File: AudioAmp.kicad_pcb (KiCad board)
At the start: 2 copper layers, 60.1 x 56.5 mm, 10 parts, among them J1 Conn_01x02, J2 Conn_01x02, J3 Conn_01x02, U1 LM386

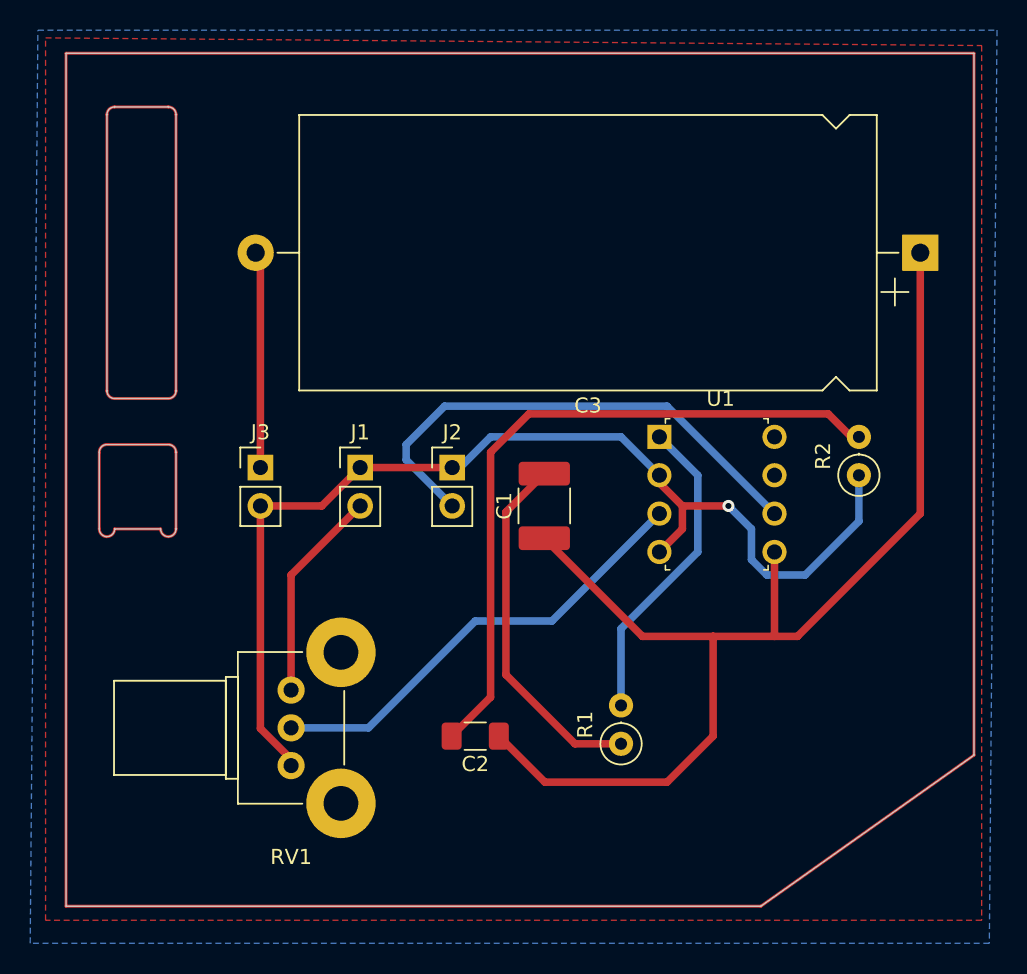
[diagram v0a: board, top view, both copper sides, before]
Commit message: Edits based on what I see
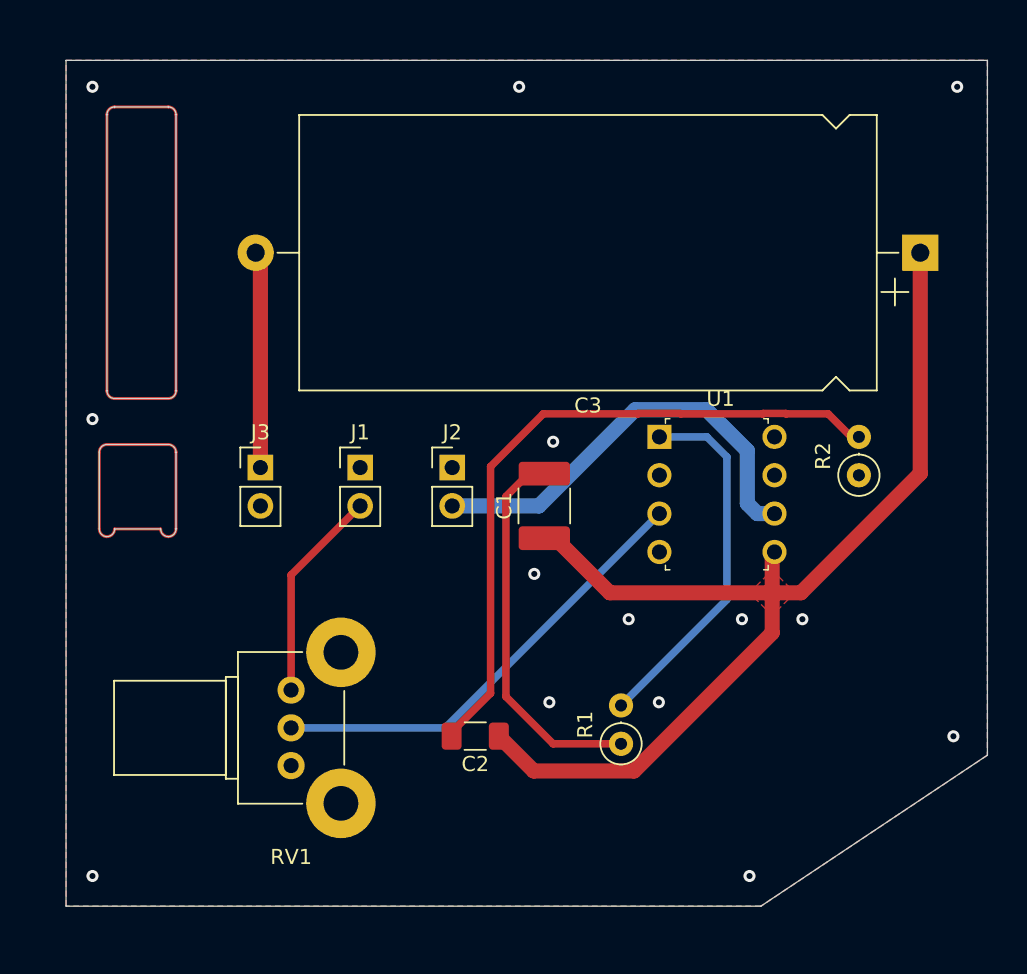
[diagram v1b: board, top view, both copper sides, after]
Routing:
- net GND: track 73.0 -> 0.94 mm, vias 1 -> 14
- net Net-(J2-Pad2): track 33.7 -> 28.9 mm
- net Net-(C1-Pad1): track 77.1 -> 72.8 mm
- net Net-(R1-Pad2): track 20.9 -> 24.4 mm
- net Net-(C1-Pad2): track 23.9 -> 25.3 mm
- net Net-(C2-Pad2): track 46.6 -> 46.1 mm
- added copper zone on F.Cu, net Net-(C1-Pad1)
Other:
- board size 60.1 x 56.5 mm -> 61 x 56 mm
- net class Default: clearance 0.2 -> 0.5; trace_width 0.25 -> 0.5; via_dia 0.8 -> 1; via_drill 0.4 -> 0.5
- net class Power added: clearance 0.5, trace_width 1, via_dia 2, via_drill 1
- rule trace_clearance: 0.2 -> 0.5
